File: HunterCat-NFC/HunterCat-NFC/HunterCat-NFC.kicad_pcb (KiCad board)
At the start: 2 copper layers, 112 x 33.5 mm, 74 parts, among them J1 Battery, J2 Conn_01x06_Female, P1 USB_C_Plug_USB2.0, Q1 DMG3415U-7, SW1 RESET, SW2 GPIO, SW3 GPIO1, SW4 GPIO2, U1 ATSAMD21E18A, U2 PN7150B0HN_C11002E-PN7150B0HN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, U3 MCP73831-3-OT, U4 AP2112K-3.3, U5 GD25Q16CEIGR, Y1 27.12Mhz

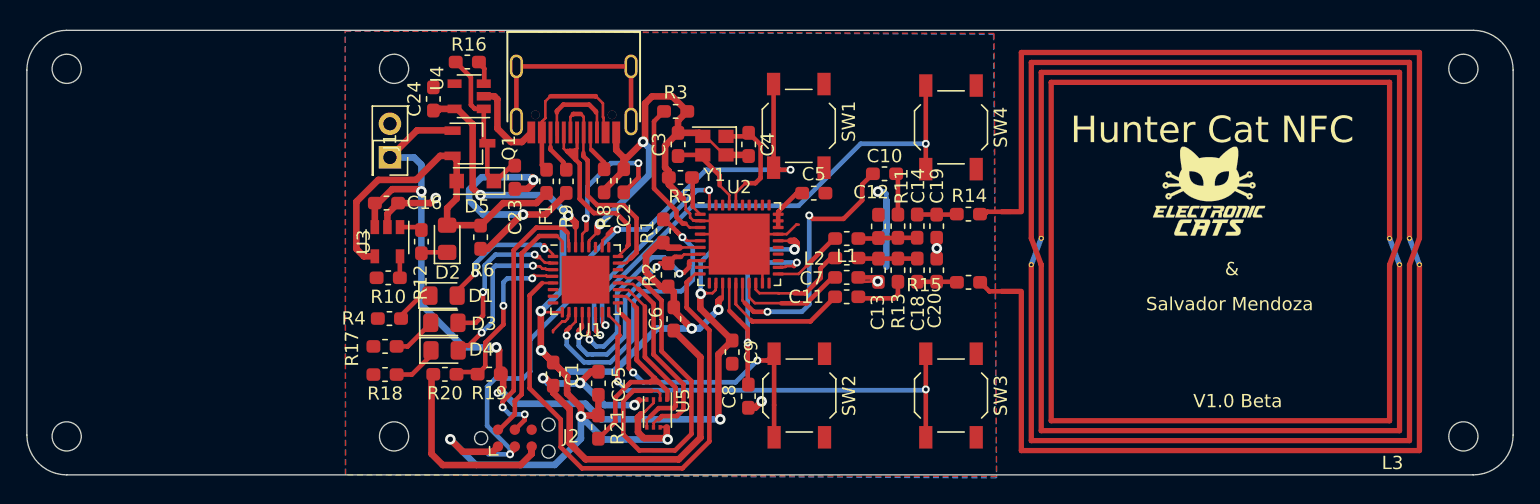
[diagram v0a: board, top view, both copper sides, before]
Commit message: new size
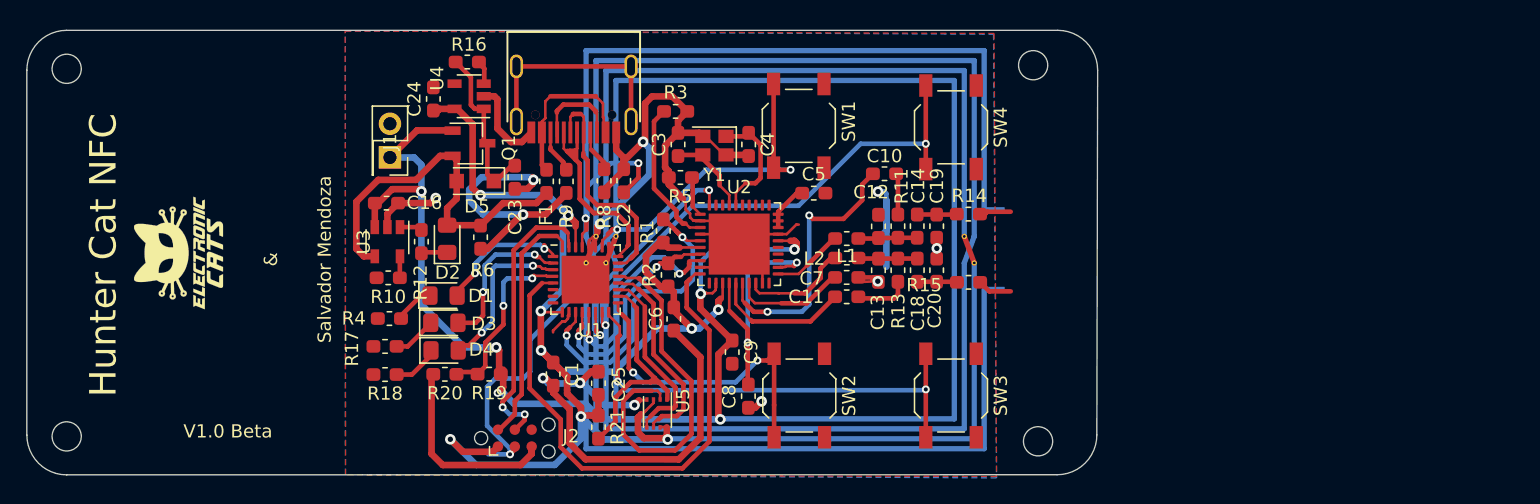
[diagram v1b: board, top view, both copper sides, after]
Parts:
- removed the REF** at (107.7, 106.1)
- removed the REF** at (107.7, 78.4)
- L3: moved to B.Cu
- moved G*** 77.8 mm to (91.4, 92.3), turned to 90 degrees
- moved svg2mod 48.0 mm to (101.9, 94.2)
- moved L3 32.8 mm to (137.1, 92.0), turned to 180 degrees
- moved REF** 32.4 mm to (155.8, 78.1)
- moved REF** 32.1 mm to (156.2, 106.5)
- moved REF** 18.5 mm to (151.3, 92.9)
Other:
- board size 112 x 33.5 mm -> 80.7 x 33.5 mm

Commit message: Change ant
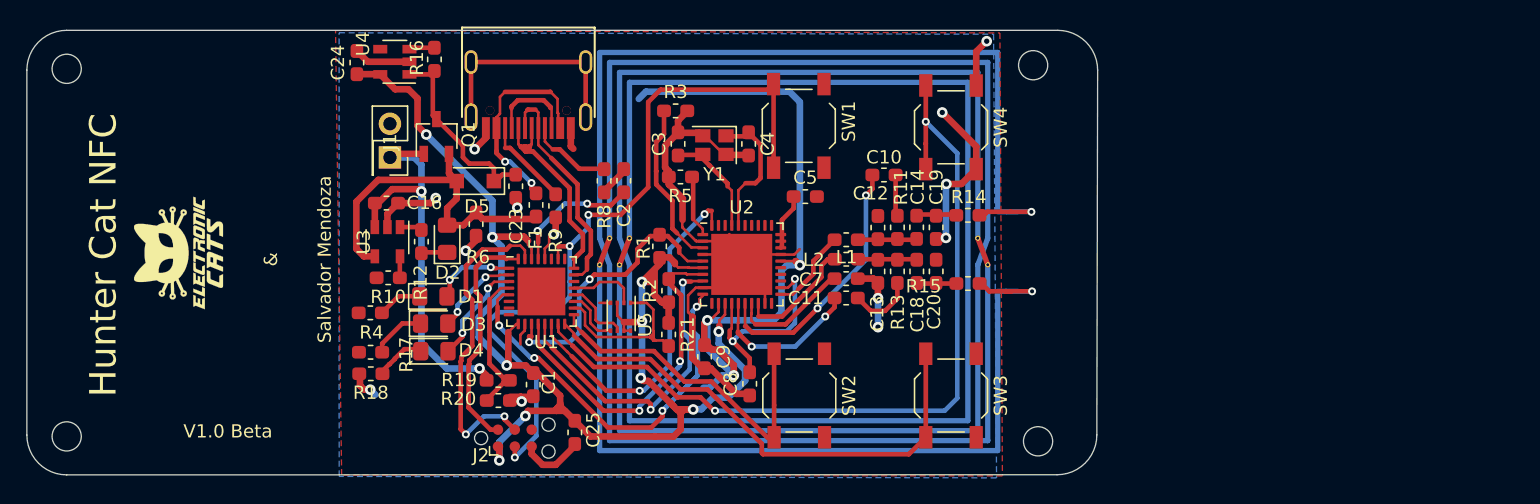
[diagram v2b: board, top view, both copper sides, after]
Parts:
- removed C6: 1uF, Capacitor_SMD:C_0603_1608Metric_Pad1.05x0.95mm_HandSolder
- moved R21 8.76 mm to (128.4, 98.4)
- moved U5 7.78 mm to (125.5, 96.0)
- moved C24 6.38 mm to (104.9, 77.9)
- moved U4 6.17 mm to (107.7, 77.9)
- moved R20 4.49 mm to (115.5, 103.4), turned to 0 degrees
- moved C25 4.11 mm to (121.3, 105.8), turned to 270 degrees
- moved U1 3.44 mm to (118.8, 95.2)
- moved P1 3.44 mm to (117.8, 82.0)
- moved Q1 2.58 mm to (110.9, 83.5), turned to 90 degrees
- moved R16 2.49 mm to (110.7, 77.7), turned to 90 degrees
- moved C9 2.11 mm to (131.1, 100.1)
- moved R9 2.02 mm to (119.8, 88.7)
- moved F1 1.95 mm to (118.4, 88.7)
- moved C1 1.70 mm to (118.2, 102.2)
- moved U2 1.54 mm to (133.9, 93.1)
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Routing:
- net GND: track 162.3 -> 107.2 mm, vias 12 -> 13
- net /GPIO2: track 38.9 -> 61.6 mm
- net /MISO: track 27.5 -> 5.25 mm
- net /SCK: track 15.2 -> 5.07 mm
- net /MOSI: track 14.2 -> 4.42 mm
- net /SCL: track 17.0 -> 25.5 mm
- net /CLK: track 18.7 -> 26.8 mm
- net /IRQ: track 16.4 -> 24.4 mm
- net /RST: track 49.9 -> 56.8 mm
- net /VEN: track 41.3 -> 35.0 mm, vias 0 -> 4
- net +BATT: track 77.2 -> 82.8 mm, vias 6 -> 5
- net /LED2: track 11.7 -> 6.52 mm
- net /LED3: track 12.3 -> 7.80 mm
- net Net-(L3-Pad2): track 2.59 -> 6.56 mm, vias 0 -> 1
- net /LED1: track 10.3 -> 6.69 mm
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
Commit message: last revision
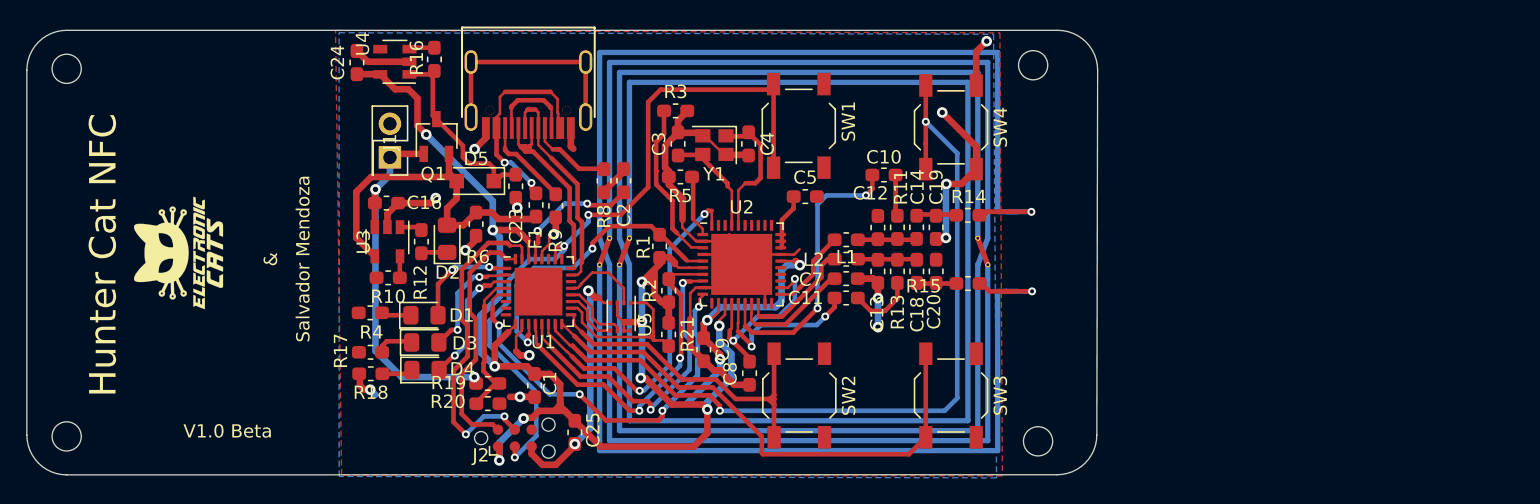
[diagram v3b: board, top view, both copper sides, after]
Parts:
- moved D1 1.57 mm to (110.0, 97.0)
- moved D3 1.57 mm to (110.0, 99.0)
- moved D4 1.57 mm to (110.0, 101.1)
- moved R20 0.82 mm to (114.7, 103.6)
- moved R19 0.82 mm to (114.7, 102.1)
- moved C8 0.80 mm to (134.5, 101.3)
- moved C9 0.53 mm to (131.0, 99.6)
- moved U1 0.22 mm to (118.6, 95.2)
- moved C1 0.12 mm to (118.3, 102.3)
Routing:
- net +BATT: track 82.8 -> 50.9 mm
- net GND: track 107.2 -> 121.1 mm, vias 13 -> 16
- net /LED2: track 6.52 -> 9.02 mm
- net /LED3: track 7.80 -> 9.92 mm
- net /LED1: track 6.69 -> 8.68 mm
- net Net-(C8-Pad1): track 16.4 -> 14.6 mm
- net /SDA: track 21.6 -> 23.4 mm
- net /RXP: track 20.3 -> 22.0 mm
- net /RST: track 56.8 -> 55.1 mm
- net Net-(D4-Pad1): track 3.89 -> 2.34 mm
- net Net-(D3-Pad1): track 4.18 -> 2.84 mm
- net +3V3: track 108.6 -> 109.9 mm
- net /SWDIO: track 17.6 -> 18.8 mm
- net Net-(D1-Pad1): track 3.37 -> 2.25 mm
- net /VEN: track 35.0 -> 36.0 mm
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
